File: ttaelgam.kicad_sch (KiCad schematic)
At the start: 222 parts, among them J1 USB_C_Receptacle_USB2.0_16P, J2 Conn_01x04, J3 Conn_01x05, U1 XC6206PxxxMR, U2 RP2040, U3 SRV05-4, U4 W25Q128JVS, Y1 Crystal_GND24

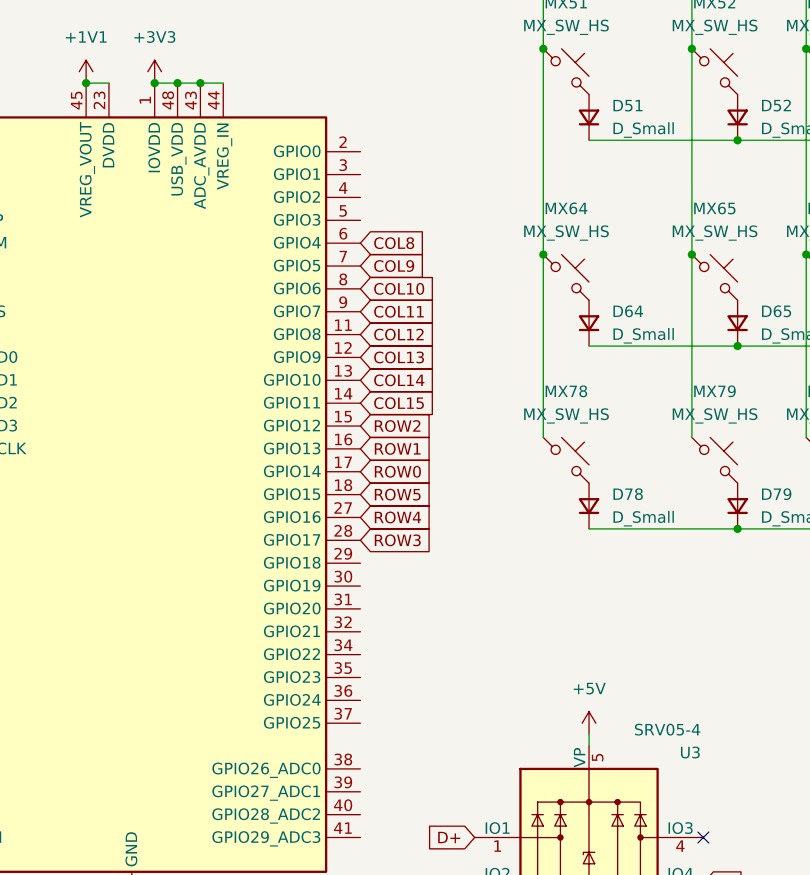
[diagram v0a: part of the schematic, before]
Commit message: 0810
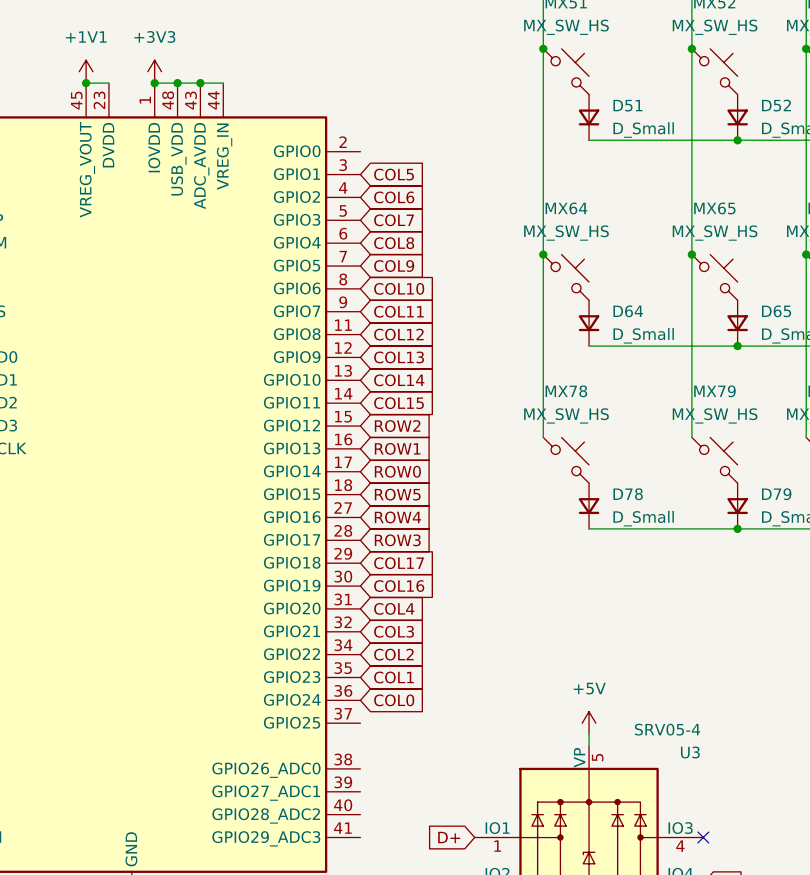
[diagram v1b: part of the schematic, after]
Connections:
- net COL0: now also U2.36 (GPIO24)
- net COL1: now also U2.35 (GPIO23)
- net COL16: now also U2.30 (GPIO19)
- net COL17: now also U2.29 (GPIO18)
- net COL2: now also U2.34 (GPIO22)
- net COL3: now also U2.32 (GPIO21)
- net COL4: now also U2.31 (GPIO20)
- net COL5: now also U2.3 (GPIO1)
- net COL6: now also U2.4 (GPIO2)
- net COL7: now also U2.5 (GPIO3)
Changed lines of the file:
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@@
+		)
+	)
+	(global_label "COL5"
+		(shape input)
+		(at 85.09 147.32 0)
+		(fields_autoplaced yes)
+		(effects
+			(font
+				(size 1.27 1.27)
+			)
+			(justify left)
+		)
+		(property "Intersheetrefs" "${INTERSHEET_REFS}"
+			(at 92.9133 147.32 0)
+			(effects
+				(font
+					(size 1.27 1.27)
+				)
+				(justify left)
+				(hide yes)
+			)
 		)
 	)
@@
 		)
 	)
+	(global_label "COL0"
+		(shape input)
+		(at 85.09 205.74 0)
+		(fields_autoplaced yes)
+		(effects
+			(font
+				(size 1.27 1.27)
+			)
+			(justify left)
+		)
+		(property "Intersheetrefs" "${INTERSHEET_REFS}"
+			(at 92.9133 205.74 0)
+			(effects
+				(font
+					(size 1.27 1.27)
+				)
+				(justify left)
+				(hide yes)
+			)
+		)
+	)
 	(global_label "Q_SEL"
 		(shape input)
@@
 		)
 	)
+	(global_label "COL3"
+		(shape input)
+		(at 85.09 198.12 0)
+		(fields_autoplaced yes)
+		(effects
+			(font
+				(size 1.27 1.27)
+			)
+			(justify left)
+		)
+		(property "Intersheetrefs" "${INTERSHEET_REFS}"
+			(at 92.9133 198.12 0)
+			(effects
+				(font
+					(size 1.27 1.27)
+				)
+				(justify left)
+				(hide yes)
+			)
+		)
+	)
 	(global_label "COL6"
 		(shape input)
@@
 		)
 	)
+	(global_label "COL4"
+		(shape input)
+		(at 85.09 195.58 0)
+		(fields_autoplaced yes)
+		(effects
+			(font
+				(size 1.27 1.27)
+			)
+			(justify left)
+		)
+		(property "Intersheetrefs" "${INTERSHEET_REFS}"
+			(at 92.9133 195.58 0)
+			(effects
+				(font
+					(size 1.27 1.27)
+				)
+				(justify left)
+				(hide yes)
+			)
+		)
+	)
 	(global_label "RESET"
 		(shape input)
@@
 		)
 	)
+	(global_label "COL1"
+		(shape input)
+		(at 85.09 203.2 0)
+		(fields_autoplaced yes)
+		(effects
+			(font
+				(size 1.27 1.27)
+			)
+			(justify left)
+		)
+		(property "Intersheetrefs" "${INTERSHEET_REFS}"
+			(at 92.9133 203.2 0)
+			(effects
+				(font
+					(size 1.27 1.27)
+				)
+				(justify left)
+				(hide yes)
+			)
+		)
+	)
 	(global_label "ROW4"
 		(shape input)
@@
 		)
 	)
+	(global_label "COL7"
+		(shape input)
+		(at 85.09 152.4 0)
+		(fields_autoplaced yes)
+		(effects
+			(font
+				(size 1.27 1.27)
+			)
+			(justify left)
+		)
+		(property "Intersheetrefs" "${INTERSHEET_REFS}"
+			(at 92.9133 152.4 0)
+			(effects
+				(font
+					(size 1.27 1.27)
+				)
+				(justify left)
+				(hide yes)
+			)
+		)
+	)
 	(global_label "COL5"
 		(shape input)
@@
 		)
 	)
+	(global_label "COL17"
+		(shape input)
+		(at 85.09 190.5 0)
+		(fields_autoplaced yes)
+		(effects
+			(font
+				(size 1.27 1.27)
+			)
+			(justify left)
+		)
+		(property "Intersheetrefs" "${INTERSHEET_REFS}"
+			(at 94.1228 190.5 0)
+			(effects
+				(font
+					(size 1.27 1.27)
+				)
+				(justify left)
+				(hide yes)
+			)
+		)
+	)
+	(global_label "COL16"
+		(shape input)
+		(at 85.09 193.04 0)
+		(fields_autoplaced yes)
+		(effects
+			(font
+				(size 1.27 1.27)
+			)
+			(justify left)
+		)
+		(property "Intersheetrefs" "${INTERSHEET_REFS}"
+			(at 94.1228 193.04 0)
+			(effects
+				(font
+					(size 1.27 1.27)
+				)
+				(justify left)
+				(hide yes)
+			)
+		)
+	)
 	(global_label "COL15"
 		(shape input)
@@
 		)
 	)
+	(global_label "COL6"
+		(shape input)
+		(at 85.09 149.86 0)
+		(fields_autoplaced yes)
+		(effects
+			(font
+				(size 1.27 1.27)
+			)
+			(justify left)
+		)
+		(property "Intersheetrefs" "${INTERSHEET_REFS}"
+			(at 92.9133 149.86 0)
+			(effects
+				(font
+					(size 1.27 1.27)
+				)
+				(justify left)
+				(hide yes)
+			)
+		)
+	)
 	(global_label "RESET"
 		(shape input)
@@
 				(hide yes)
 			)
+		)
+	)
+	(global_label "COL2"
+		(shape input)
+		(at 85.09 200.66 0)
+		(fields_autoplaced yes)
+		(effects
+			(font
+				(size 1.27 1.27)
+			)
+			(justify left)
+		)
+		(property "Intersheetrefs" "${INTERSHEET_REFS}"
+			(at 92.9133 200.66 0)
+			(effects
+				(font
+					(size 1.27 1.27)
+				)
+				(justify left)
+				(hide yes)
+			)

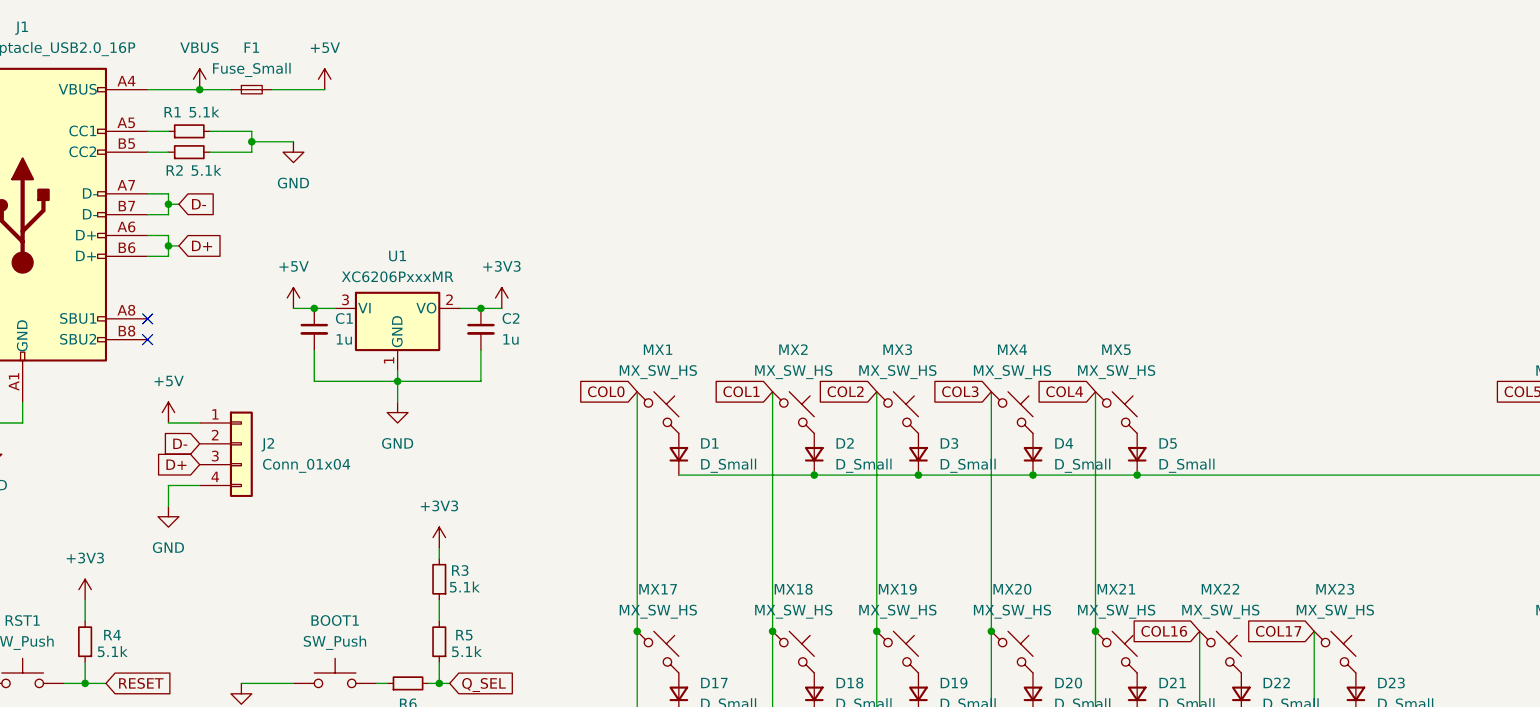
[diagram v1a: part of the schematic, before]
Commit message: 0817
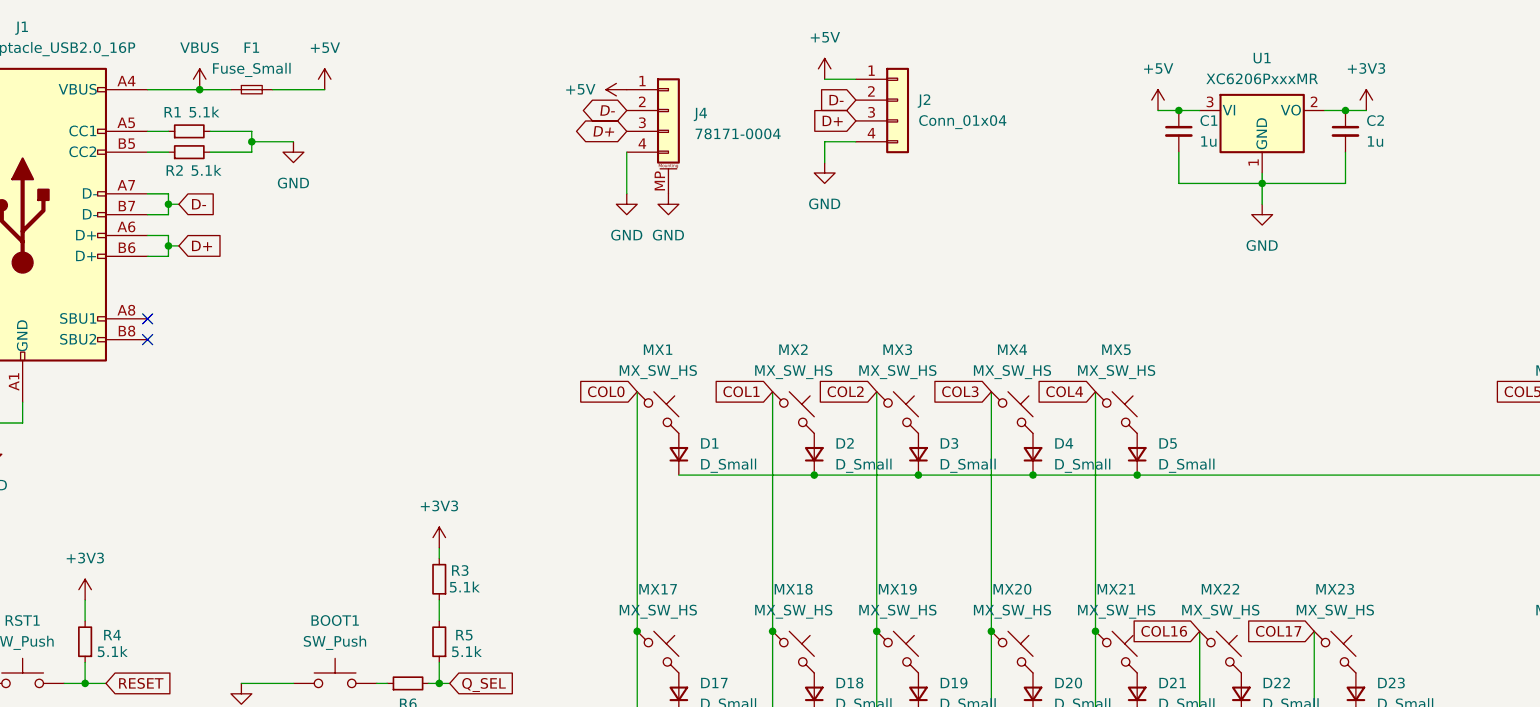
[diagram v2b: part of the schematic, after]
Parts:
- added J4: 78171-0004, Connector_Molex:Molex_Pico-EZmate_78171-0004_1x04-1MP_P1.20mm_Vertical, symbol Connector_Generic_MountingPin:Conn_01x04_MountingPin
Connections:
- net +5V: now also J4.1 (Pin_1)
- net D+: now also J4.3 (Pin_3)
- net D-: now also J4.2 (Pin_2)
- net GND: now also J4.4 (Pin_4), J4.MP (MountPin)
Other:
- moved on the sheet: C1, C2, J2, U1

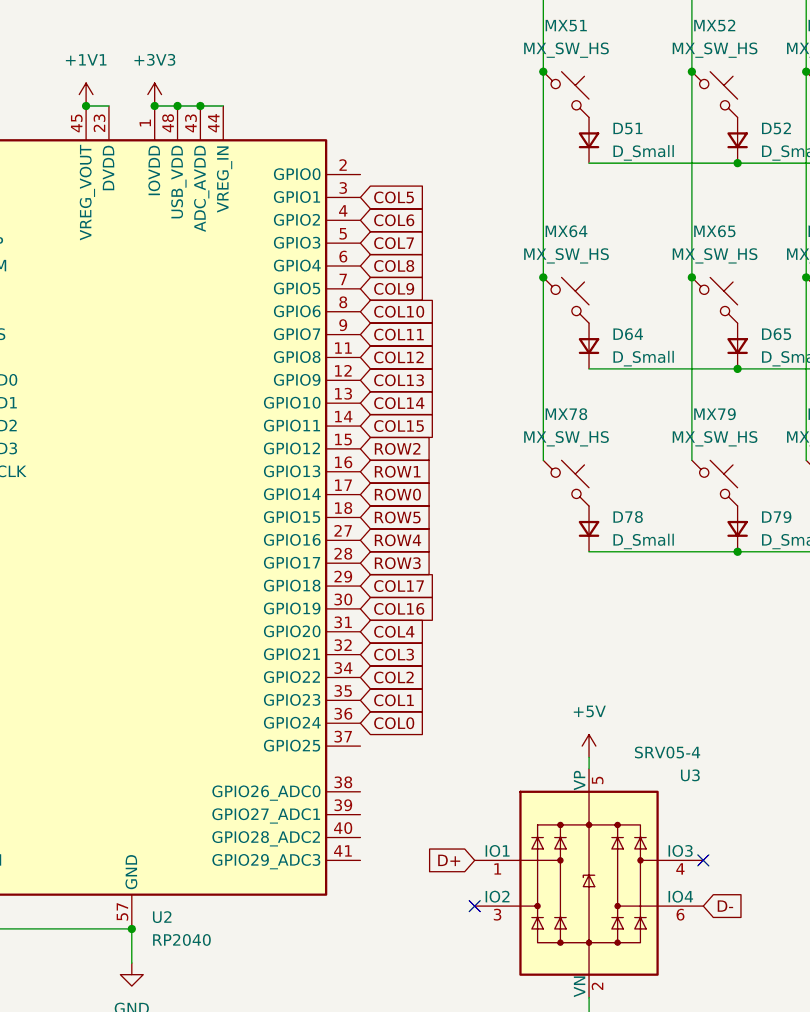
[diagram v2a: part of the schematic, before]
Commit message: 0901
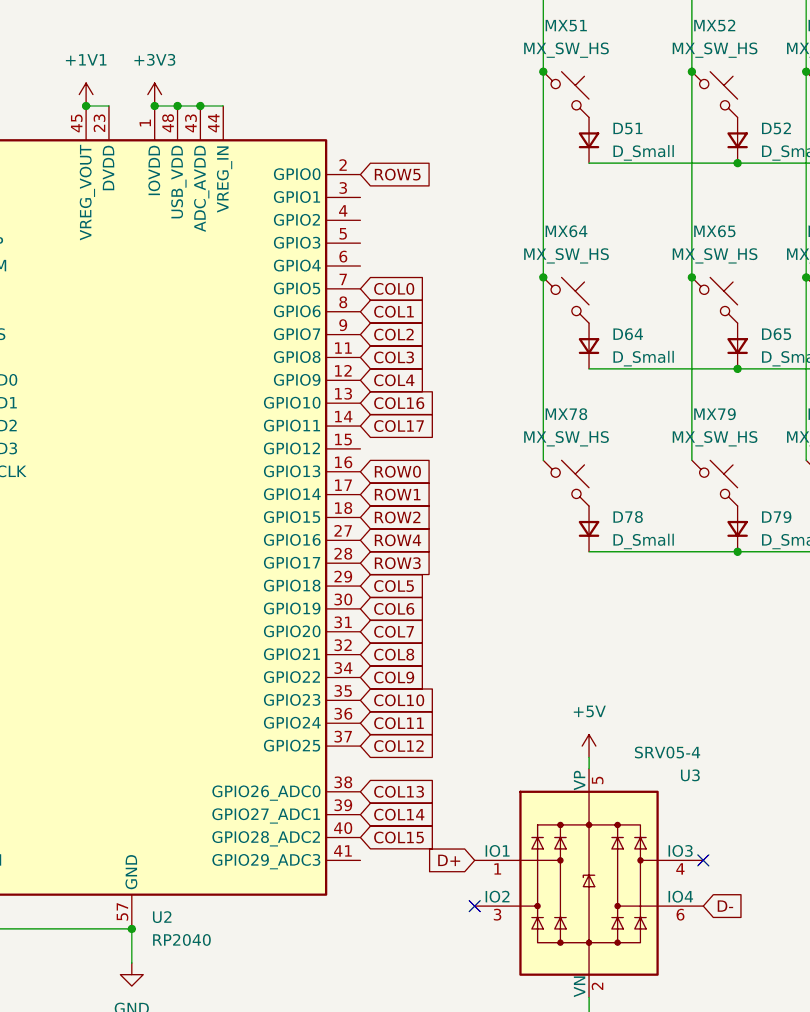
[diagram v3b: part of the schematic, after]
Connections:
- net COL0: now also U2.7 (GPIO5); no longer U2.36 (GPIO24)
- net COL1: now also U2.8 (GPIO6); no longer U2.35 (GPIO23)
- net COL10: now also U2.35 (GPIO23); no longer U2.8 (GPIO6)
- net COL11: now also U2.36 (GPIO24); no longer U2.9 (GPIO7)
- net COL12: now also U2.37 (GPIO25); no longer U2.11 (GPIO8)
- net COL13: now also U2.38 (GPIO26_ADC0); no longer U2.12 (GPIO9)
- net COL14: now also U2.39 (GPIO27_ADC1); no longer U2.13 (GPIO10)
- net COL15: now also U2.40 (GPIO28_ADC2); no longer U2.14 (GPIO11)
- net COL16: now also U2.13 (GPIO10); no longer U2.30 (GPIO19)
- net COL17: now also U2.14 (GPIO11); no longer U2.29 (GPIO18)
- net COL2: now also U2.9 (GPIO7); no longer U2.34 (GPIO22)
- net COL3: now also U2.11 (GPIO8); no longer U2.32 (GPIO21)
- net COL4: now also U2.12 (GPIO9); no longer U2.31 (GPIO20)
- net COL5: now also U2.29 (GPIO18); no longer U2.3 (GPIO1)
- net COL6: now also U2.30 (GPIO19); no longer U2.4 (GPIO2)
- net COL7: now also U2.31 (GPIO20); no longer U2.5 (GPIO3)
- net COL8: now also U2.32 (GPIO21); no longer U2.6 (GPIO4)
- net COL9: now also U2.34 (GPIO22); no longer U2.7 (GPIO5)
- net ROW0: now also U2.16 (GPIO13); no longer U2.17 (GPIO14)
- net ROW1: now also U2.17 (GPIO14); no longer U2.16 (GPIO13)
- net ROW2: now also U2.18 (GPIO15); no longer U2.15 (GPIO12)
- net ROW5: now also U2.2 (GPIO0); no longer U2.18 (GPIO15)
